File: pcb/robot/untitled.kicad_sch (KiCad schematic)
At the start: 1 part

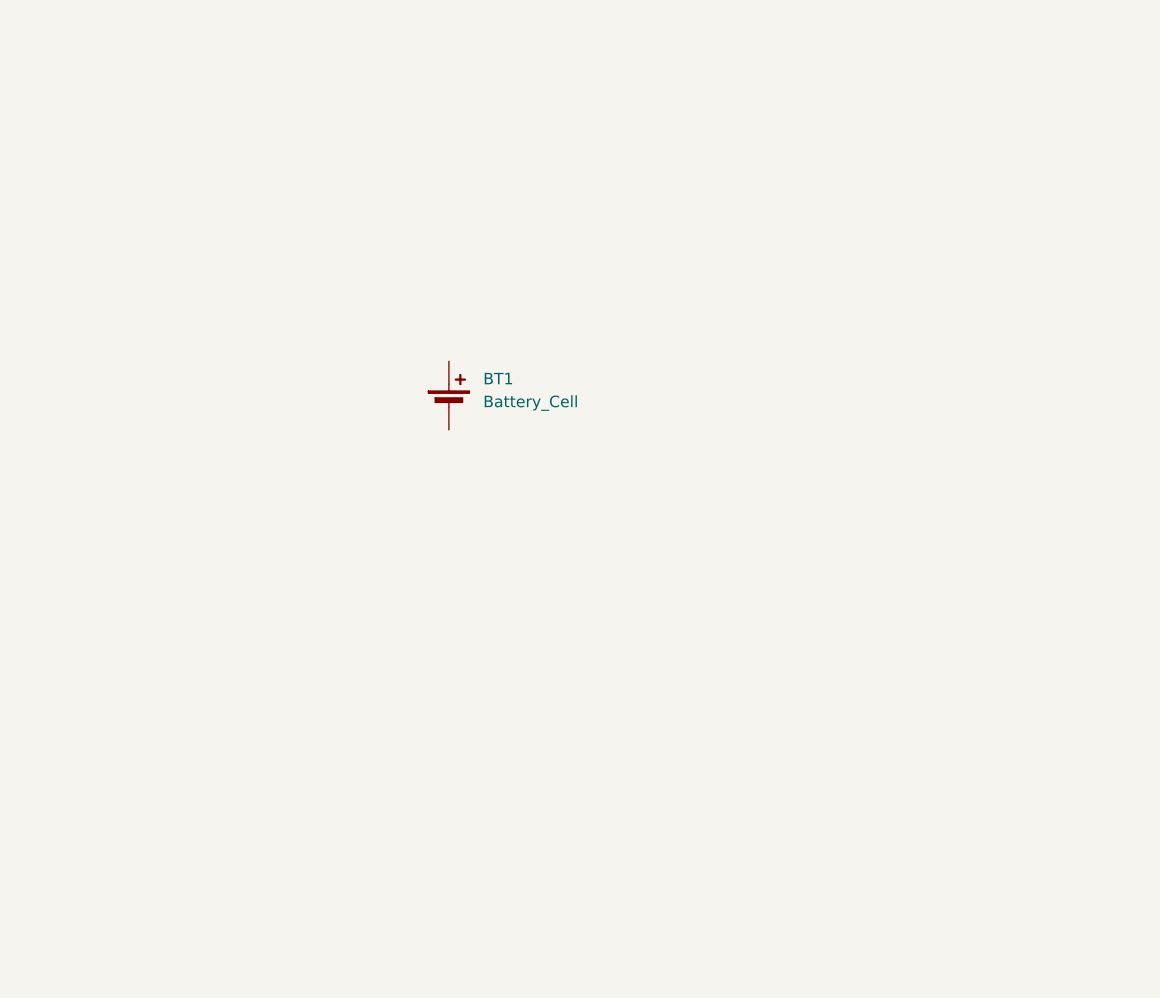
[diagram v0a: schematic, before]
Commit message: 30.1.2025 no big changes, going to get latex runing
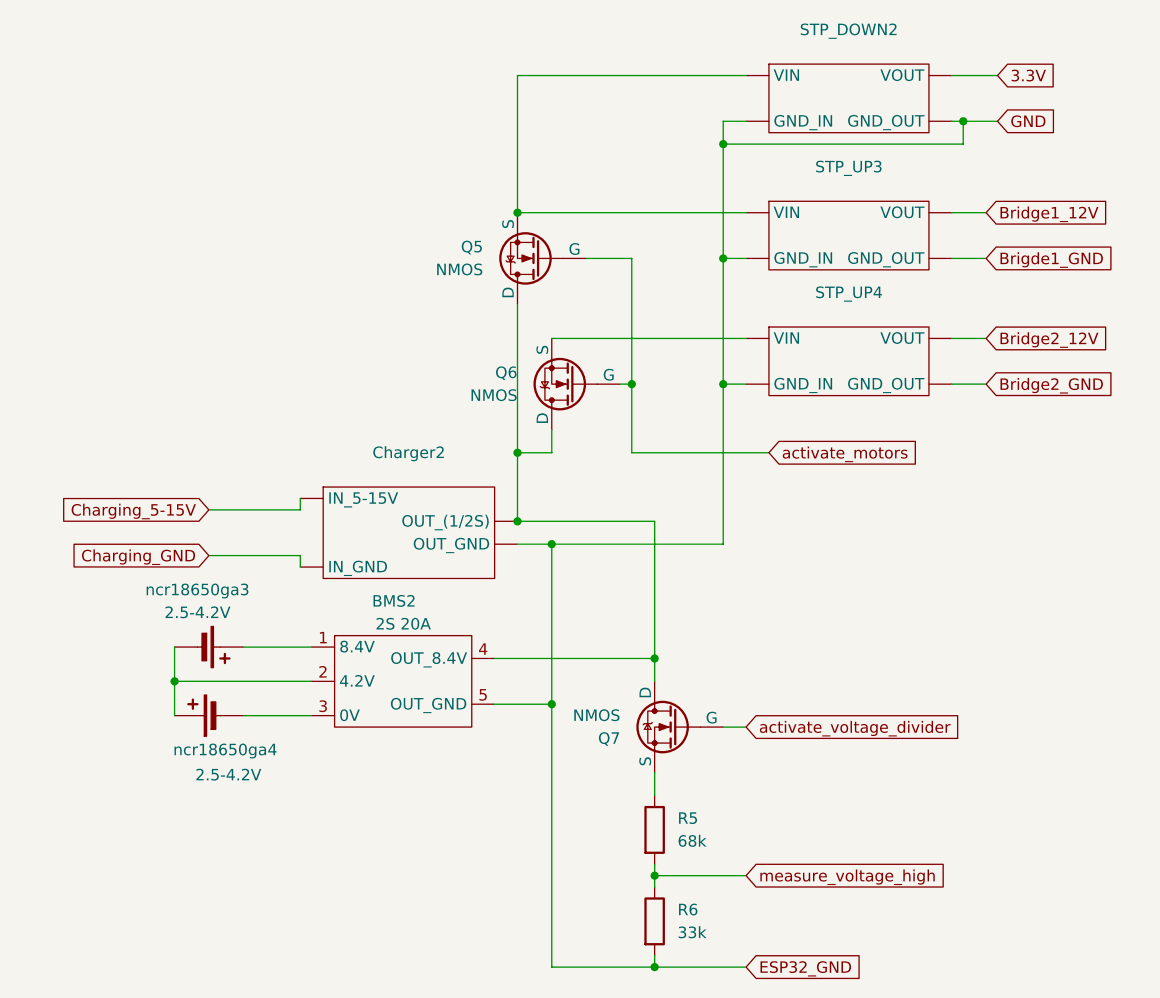
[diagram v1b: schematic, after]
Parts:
- removed BT1: Battery_Cell, symbol Device:Battery_Cell
- added BMS2: 2S 20A, symbol personalized_symbols:HW-391
- added Charger2: ~, symbol personalized_symbols:TP5100
- added Q5, Q6, Q7: NMOS, symbol Simulation_SPICE:NMOS
- added R5: 68k, symbol Device:R
- added R6: 33k, symbol Device:R
- added STP_DOWN2: ~, symbol personalized_symbols:Step_down
- added STP_UP3, STP_UP4: ~, symbol personalized_symbols:Step_Up
- added ncr18650ga3, ncr18650ga4: 2.5-4.2V, symbol Device:Battery_Cell
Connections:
- new net: Q7.3 (S), R5.1
- new net: Q6.3 (S), STP_UP4. (VOUT)
- new net: Q5.3 (S), STP_DOWN2. (VOUT), STP_UP3. (VOUT)
- new net: BMS2.4 (OUT_8.4V), Charger2. (OUT_GND), Q5.1 (D), Q6.1 (D), Q7.1 (D)
- new net: BMS2.1 (8.4V), ncr18650ga3.1 (+)
- new net: BMS2.2 (4.2V), ncr18650ga3.2 (-), ncr18650ga4.1 (+)
- new net: BMS2.3 (0V), ncr18650ga4.2 (-)
- new net 3.3V: STP_DOWN2. (VOUT)
- new net Bridge1_12V: STP_UP3. (VOUT)
- new net Bridge2_12V: STP_UP4. (VOUT)
- new net Bridge2_GND: STP_UP4. (VOUT)
- new net Brigde1_GND: STP_UP3. (VOUT)
- new net Charging_5-15V: Charger2. (OUT_GND)
- new net Charging_GND: Charger2. (OUT_GND)
- new net ESP32_GND: BMS2.5 (OUT_GND), Charger2. (OUT_GND), R6.2, STP_DOWN2. (VOUT), STP_UP3. (VOUT), STP_UP4. (VOUT)
- new net activate_motors: Q5.2 (G), Q6.2 (G)
- new net activate_voltage_divider: Q7.2 (G)
- new net measure_voltage_high: R5.2, R6.1
